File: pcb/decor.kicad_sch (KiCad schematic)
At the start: 10 parts

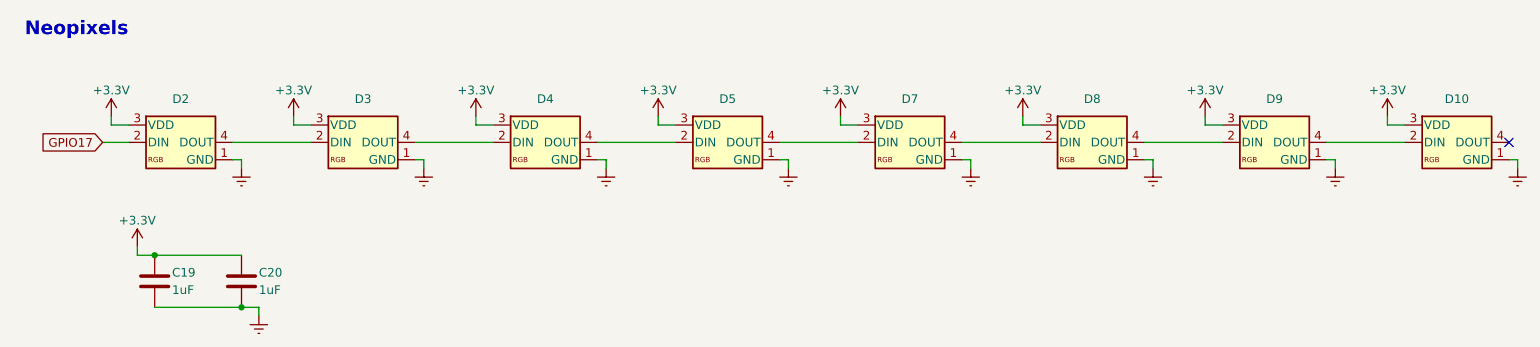
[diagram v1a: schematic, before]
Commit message: dogboard-2b3
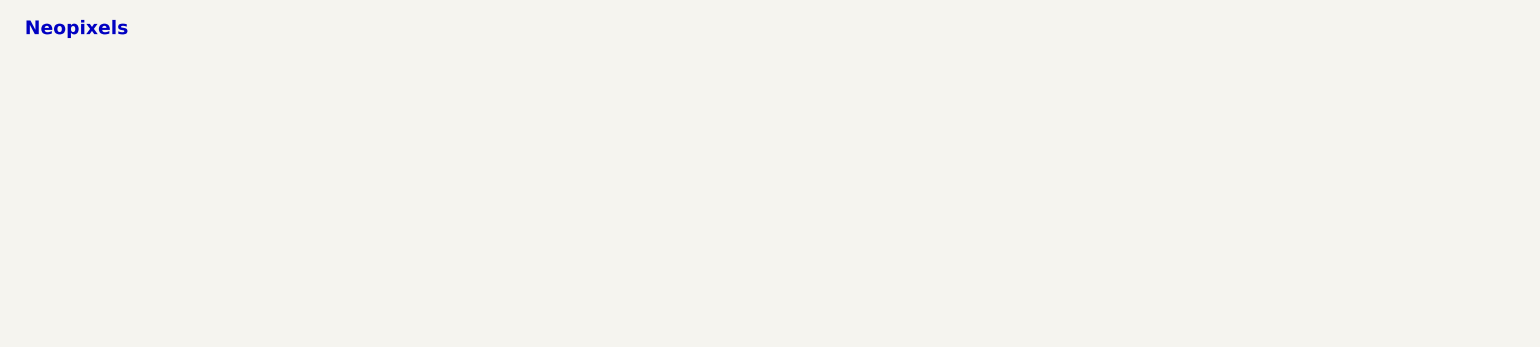
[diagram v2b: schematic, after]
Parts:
- removed C19, C20: 1uF, _custom:CAP_0603_HandSolder, symbol _custom:CAP_Standard
- removed D10, D2, D3, D4, D5, D7, D8, D9: LED_NeoPixel, _custom:LED_NeoPixel_0606, symbol _custom:LED_NeoPixel
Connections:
- no-connect marks 1 -> 0
